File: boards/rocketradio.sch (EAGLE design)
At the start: 16 parts, among them X1 BU-SMA-H

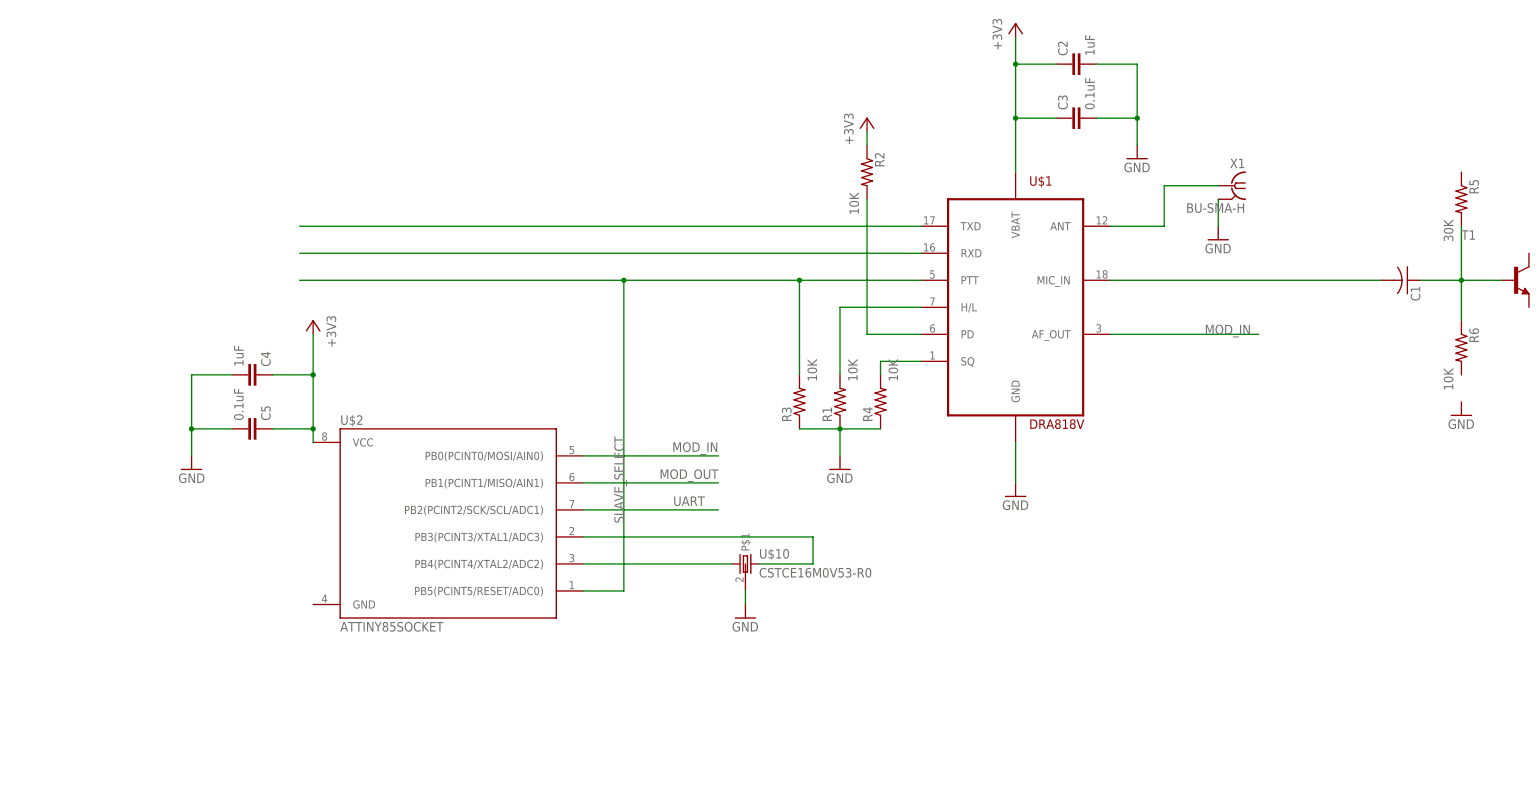
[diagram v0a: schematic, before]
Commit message: add micro
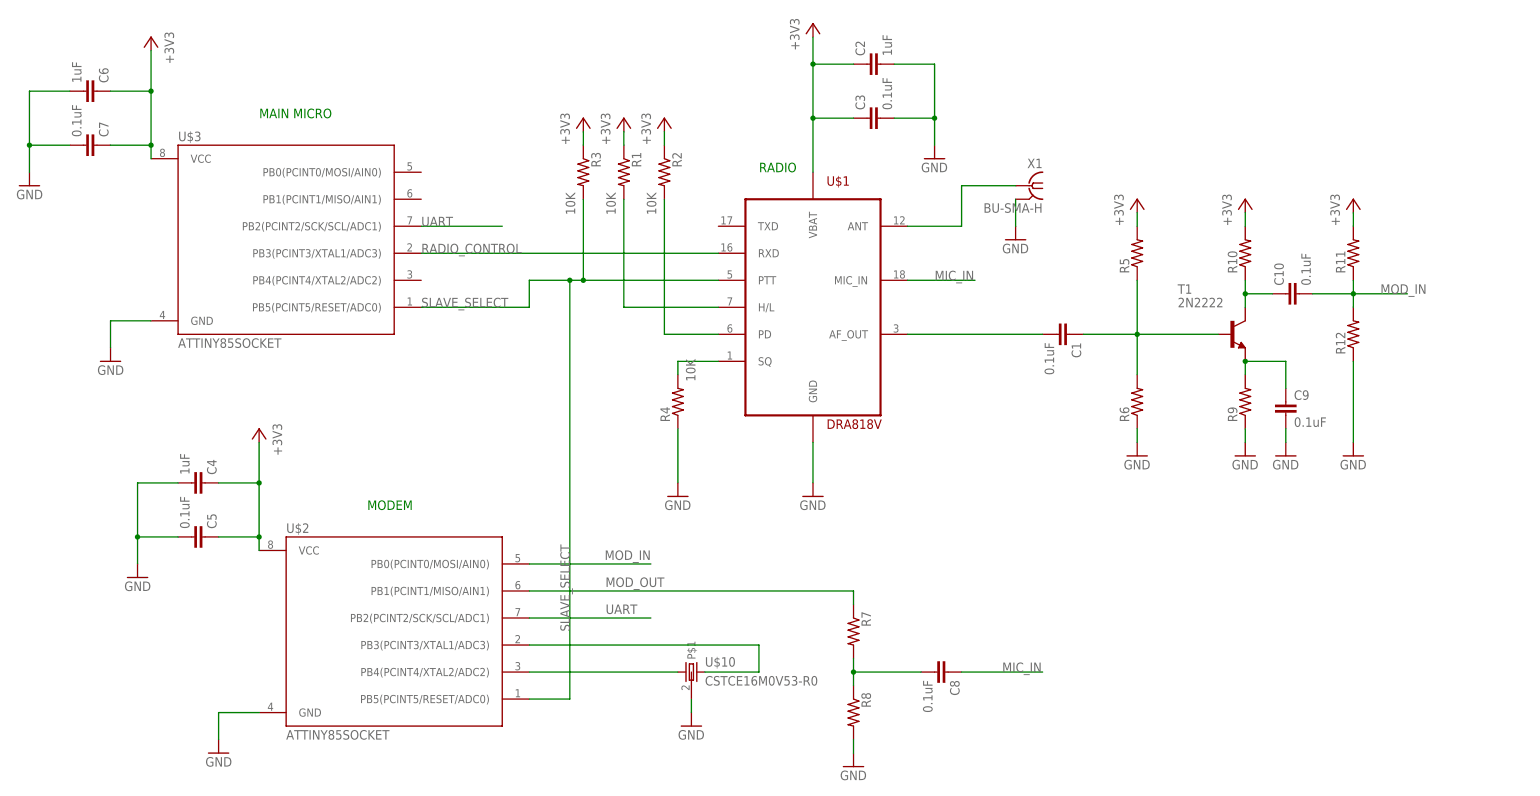
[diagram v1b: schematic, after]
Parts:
- added C10, C7, C8, C9: 0.1uF, rcl:C-EUC0603
- added C6: 1uF, rcl:C-EUC0603
- added R10, R11, R12, R7, R8, R9: (no value), rcl:R-US_R0603
- added U$3: ATTINY85SOCKET, evan:ATTINY85SOCKET
- C1: value (none) -> 0.1uF; device rcl:C-USC0603 -> rcl:C-EUC0603
- R5: value 30K -> (none)
- R6: value 10K -> (none)
- T1: value (none) -> 2N2222; device transistor:MMBT2222ALT1-NPN-SOT23-BEC -> transistor:2N2222
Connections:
- removed net N$15: U$1.RXD
- removed net N$16: U$1.TXD
- removed net N$20: C1.1, R5.2, R6.1, T1.B
- removed net N$9: C1.2, U$1.MIC_IN
- new net MIC_IN: C8.1, U$1.MIC_IN
- new net N$10: C9.1, R9.2, T1.E
- new net N$11: C10.1, R10.1, T1.C
- new net N$6: C8.2, R7.2, R8.1
- new net N$7: C1.1, R5.1, R6.2, T1.B
- new net N$8: C1.2, U$1.AF_OUT
- new net RADIO_CONTROL: U$1.RXD, U$3.PB3(PCINT3/XTAL1/ADC3)
- net +3V3: now also C6.1, C7.1, R1.1, R10.2, R11.2, R3.1, R5.2, U$3.VCC
- net GND: now also C6.2, C7.2, C9.2, R12.1, R6.1, R8.2, R9.1, U$2.GND, U$3.GND; no longer R1.1, R3.1
- net MOD_IN: now also C10.2, R11.1, R12.2; no longer U$1.AF_OUT
- net MOD_OUT: now also R7.1
- net SLAVE_SELECT: now also U$3.PB5(PCINT5/RESET/ADC0)
- net UART: now also U$3.PB2(PCINT2/SCK/SCL/ADC1)
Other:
- note added: "MAIN MICRO"
- note added: "MODEM"
- note added: "RADIO"
- moved on the sheet: C1, C2, C3, C4, C5, R1, R2, R3, R4, R5, R6, T1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
